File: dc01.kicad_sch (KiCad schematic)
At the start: 69 parts, among them J1 USB_C_Receptacle_USB2.0, J2 PROG/DEBUG, J3 Conn_01x06, J4 RJ12, J5 RJ12, J6 Conn_01x02, J7 Conn_01x02, J8 Conn_01x02, K1 AZ850-5, K2 AZ850-5, Q1 2N7002, Q2 2N7002, SW1 SW_Push, SW2 SW_Push, U1 STM32F103C8Tx, U2 AMS1117-3.3, Y1 8 MHz

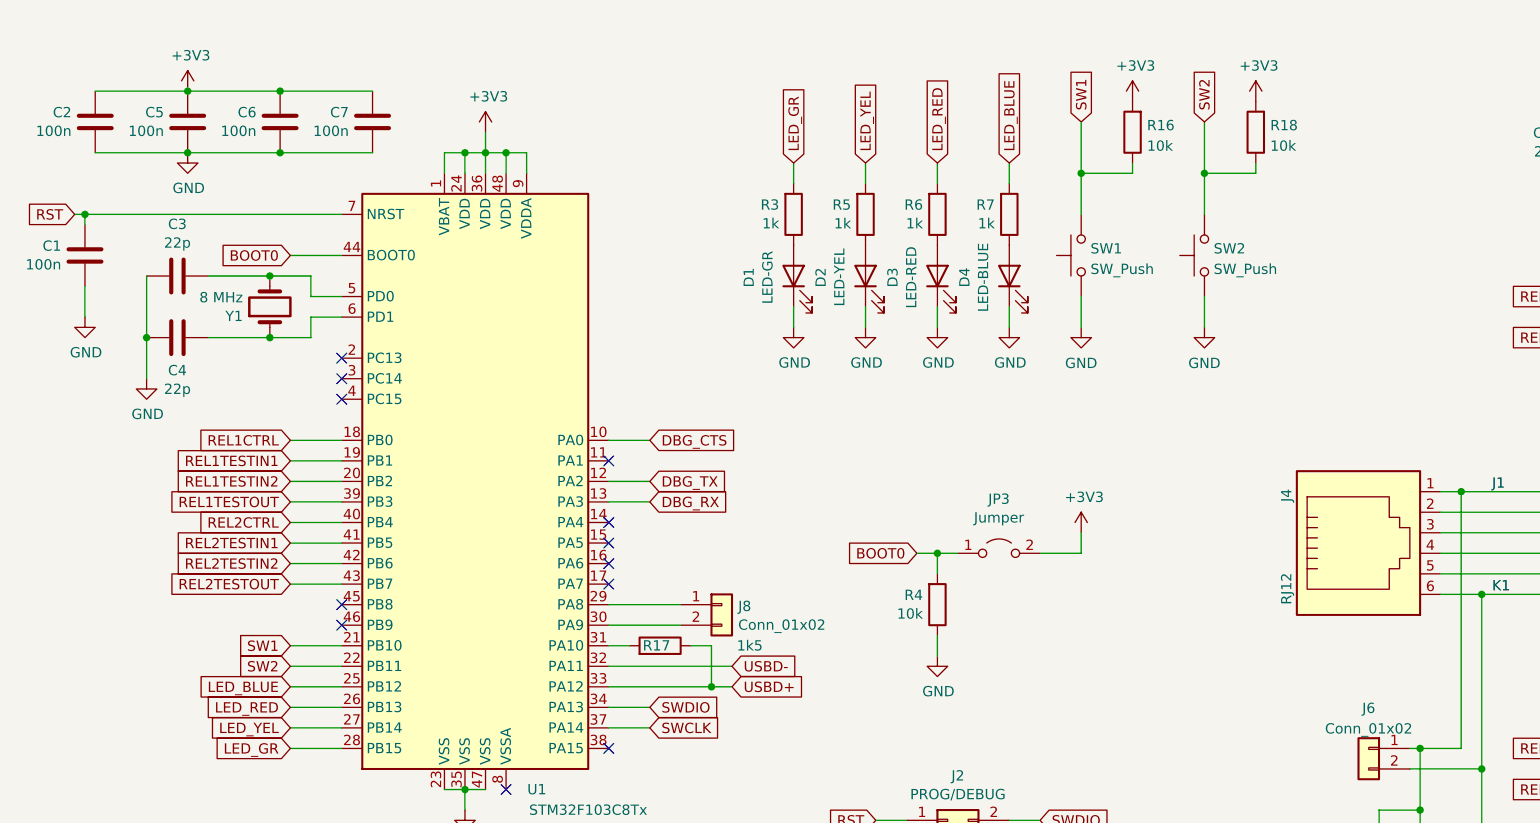
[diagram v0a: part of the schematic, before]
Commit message: Add override switch.
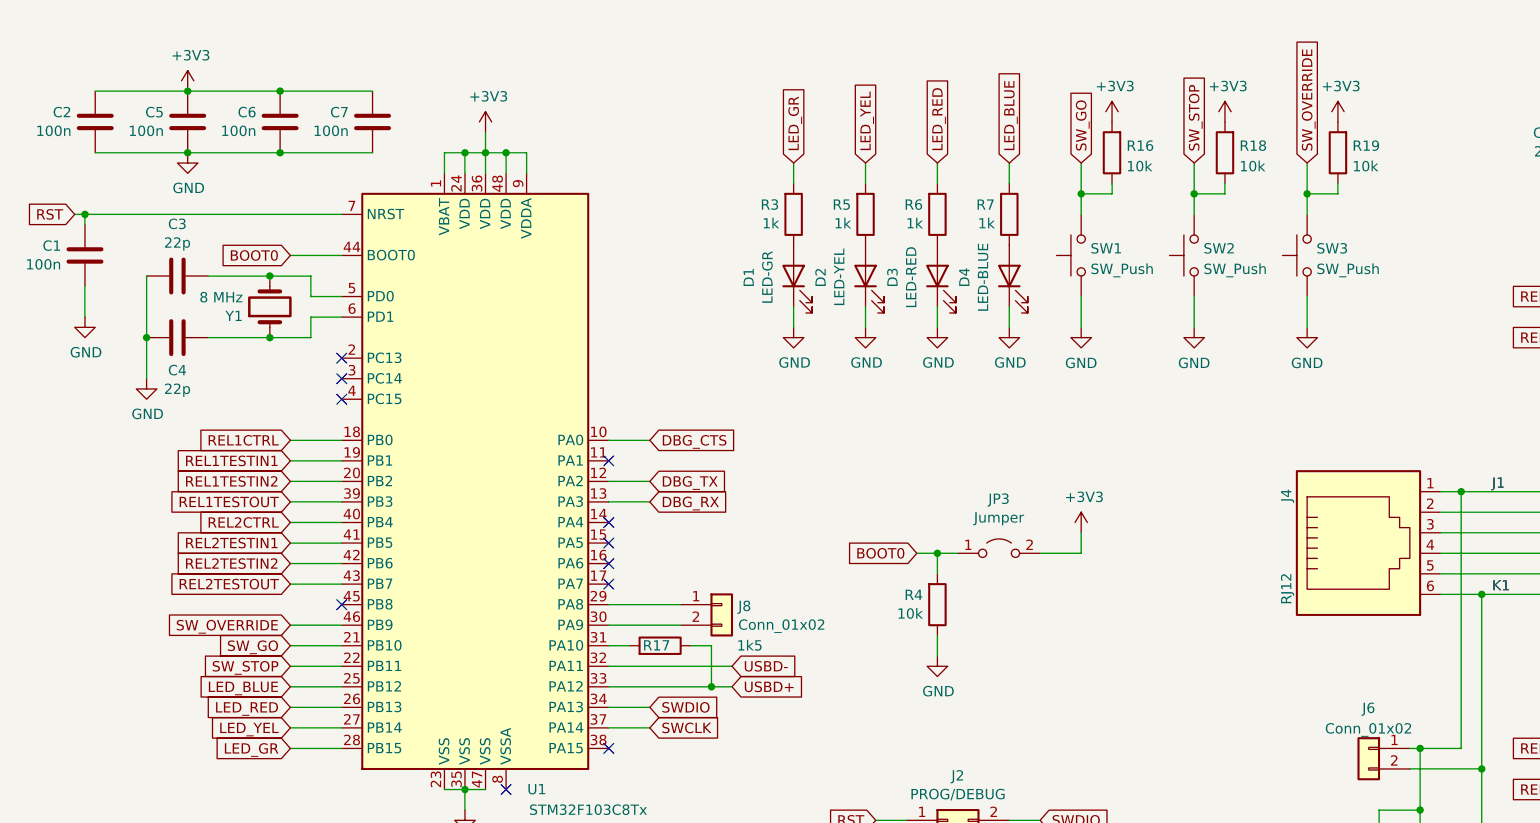
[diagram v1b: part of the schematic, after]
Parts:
- added R19: 10k, symbol Device:R
- added SW3: SW_Push, symbol Switch:SW_Push
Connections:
- net +3V3: now also R19.2
- net GND: now also SW3.1
- net SW_OVERRIDE: now reaches U1.46 (PB9)
- net SW_OVERRIDE: now also R19.1, SW3.2
- net SW1 renamed SW_GO
- net SW2 renamed SW_STOP
- no-connect marks 25 -> 24
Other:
- moved on the sheet: R16, R18, SW2

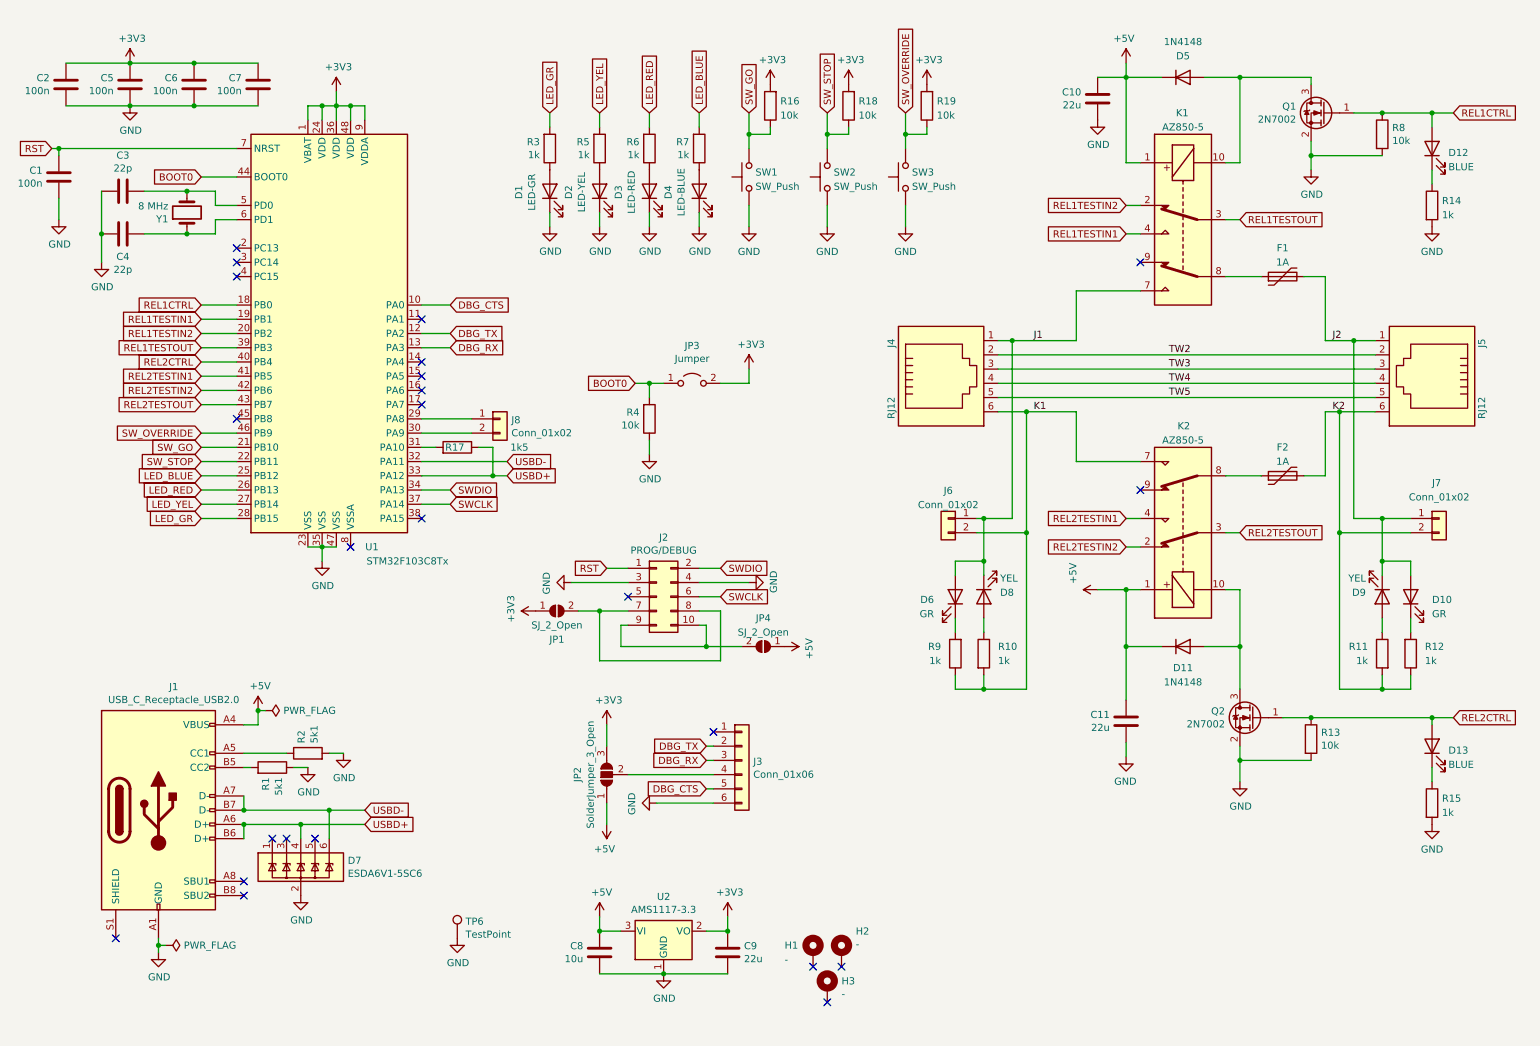
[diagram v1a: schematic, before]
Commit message: Add parts, several minor enhancements.
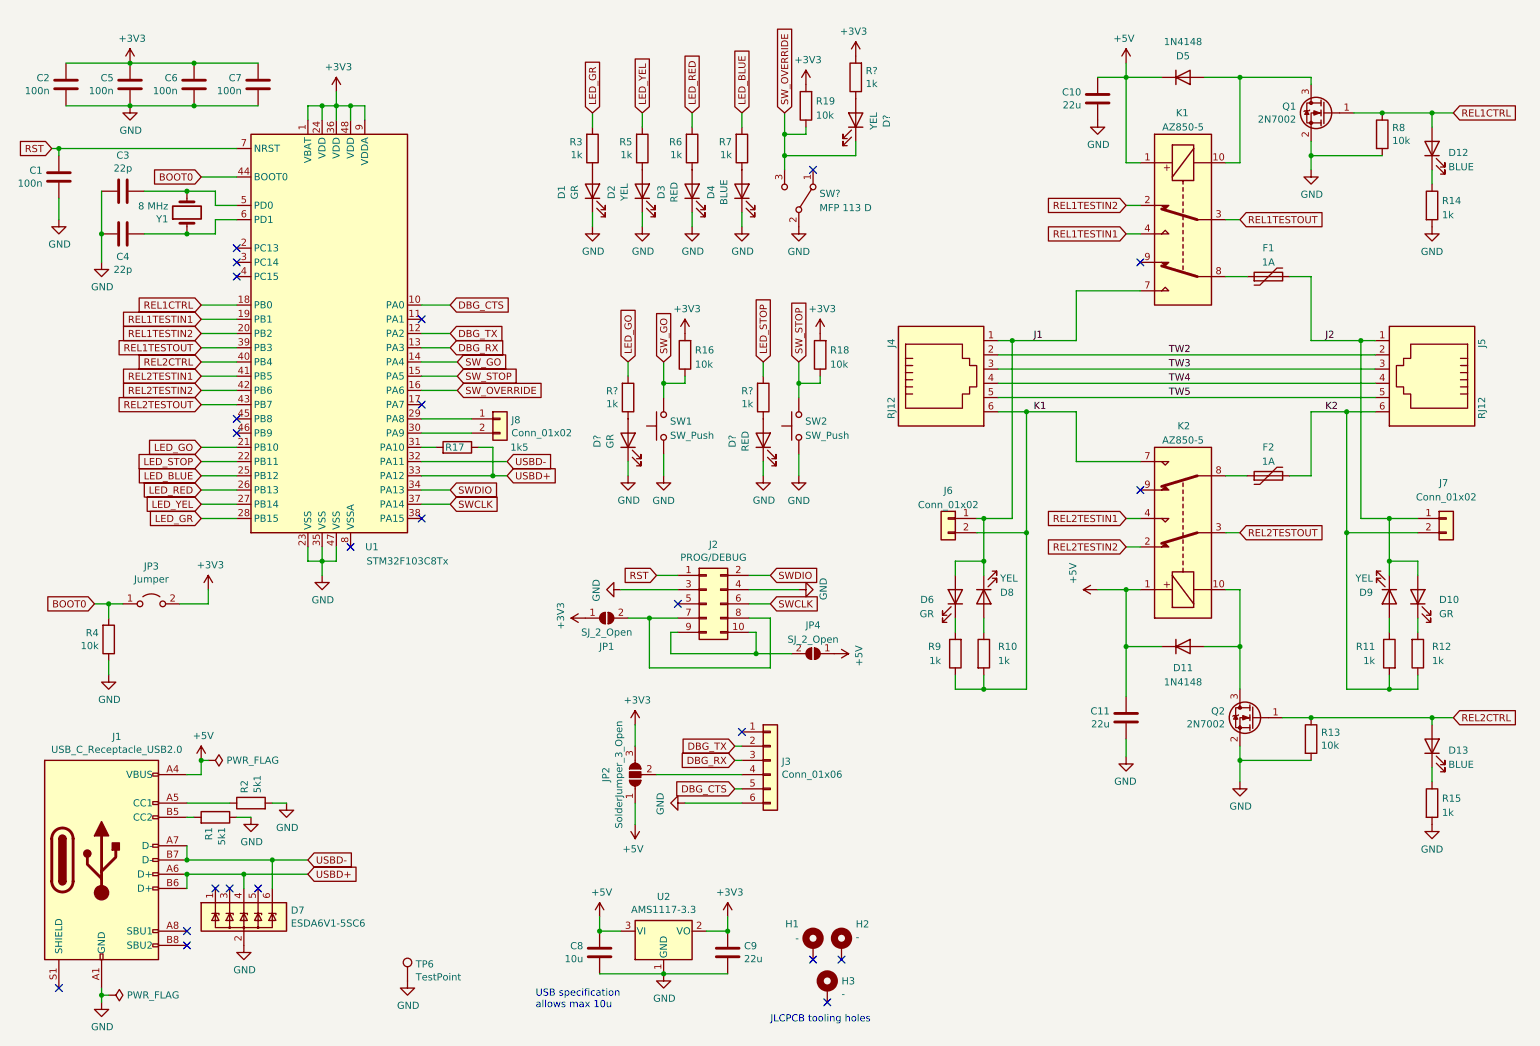
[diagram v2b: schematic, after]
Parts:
- removed SW3: SW_Push, symbol Switch:SW_Push
- added D?: YEL, LED_SMD:LED_0805_2012Metric, symbol Device:LED
- added D?: RED, LED_SMD:LED_0805_2012Metric, symbol Device:LED
- added D?: GR, LED_SMD:LED_0805_2012Metric, symbol Device:LED
- added R? (x3): 1k, Resistor_SMD:R_0805_2012Metric, symbol Device:R
- added SW?: MFP 113 D, Button_Switch_THT:SW_Slide_1P2T_CK_OS102011MS2Q, symbol Switch:SW_SPDT
- D1: value LED-GR -> GR
- D10, D12, D13, D6, D8, D9: footprint (none) -> LED_SMD:LED_0805_2012Metric
- D2: value LED-YEL -> YEL
- D3: value LED-RED -> RED
- D4: value LED-BLUE -> BLUE
- F1, F2: footprint (none) -> Fuse:Fuse_1206_3216Metric
- R10, R11, R12, R14, R15, R16, R18, R19, R9: footprint (none) -> Resistor_SMD:R_0805_2012Metric
- SW1, SW2: footprint (none) -> Button_Switch_THT:SW_PUSH_6mm_H4.3mm
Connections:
- net +3V3: now also R?.2
- net GND: now also D?.1 (K), D?.1 (K), SW?.2 (B)
- net SW_GO: now also U1.14 (PA4); no longer U1.21 (PB10)
- net SW_OVERRIDE: now also U1.16 (PA6), D?.1 (K), SW?.3 (C); no longer U1.46 (PB9)
- net SW_STOP: now also U1.15 (PA5); no longer U1.22 (PB11)
- new net: D?.2 (A), R?.1 (x3)
- new net LED_GO: R?.2, U1.21 (PB10)
- new net LED_STOP: R?.2, U1.22 (PB11)
- no-connect marks 24 -> 23
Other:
- note added: "JLCPCB tooling holes"
- note added: "USB specification allows max 10u"
- moved on the sheet: C11, D1, D10, D2, D3, D4, D7, D9, F1, F2, H1, H2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
